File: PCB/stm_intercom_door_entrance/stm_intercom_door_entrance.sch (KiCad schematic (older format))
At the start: 48 parts, among them J1 Conn_01x02, J10 Conn_01x02, J11 Conn_01x04, J12 Conn_01x04, J13 Conn_01x04, J14 Conn_01x02, J15 Conn_01x02, J16 Conn_01x01, J17 Conn_01x03, J18 Conn_01x03, J19 Conn_01x03, J2 Conn_01x04, J3 Conn_01x04, J4 Conn_01x02, J5 Conn_01x04, J6 Conn_01x02, J7 Conn_01x02, J8 Conn_01x04, J9 Conn_01x04, K1 SANYOU_SRD_Form_C, K2 SANYOU_SRD_Form_C, Q1 2N2219, Q2 2N2219, U1 YAAJ_BluePill_Part_Like, U2 MCP2551-I-P, U3 MAX3232_convertor, U4 4N25, U5 L7805, U6 4N25

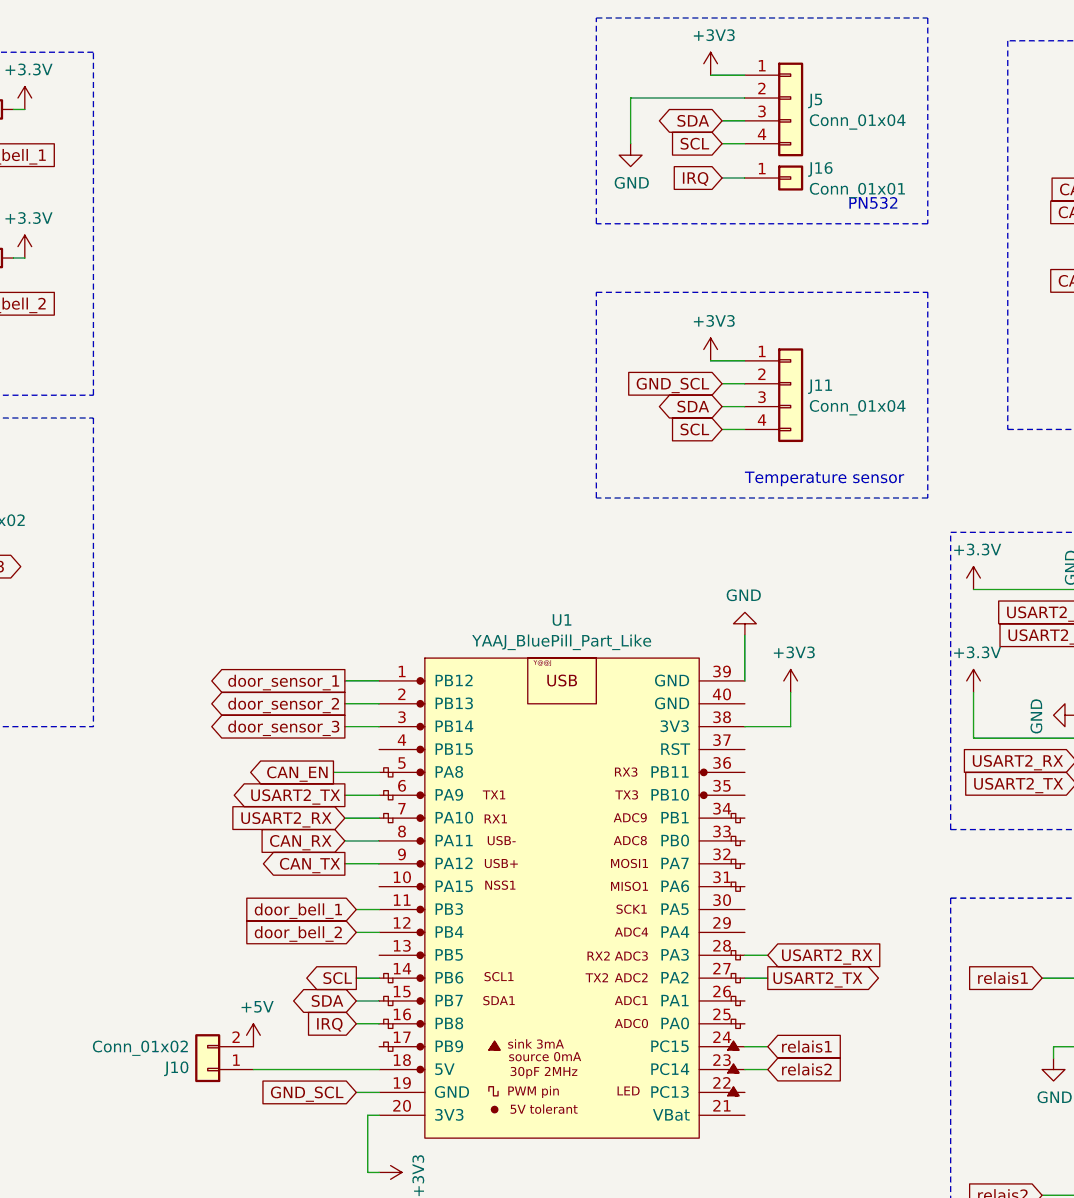
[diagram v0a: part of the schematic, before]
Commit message: Update schematic
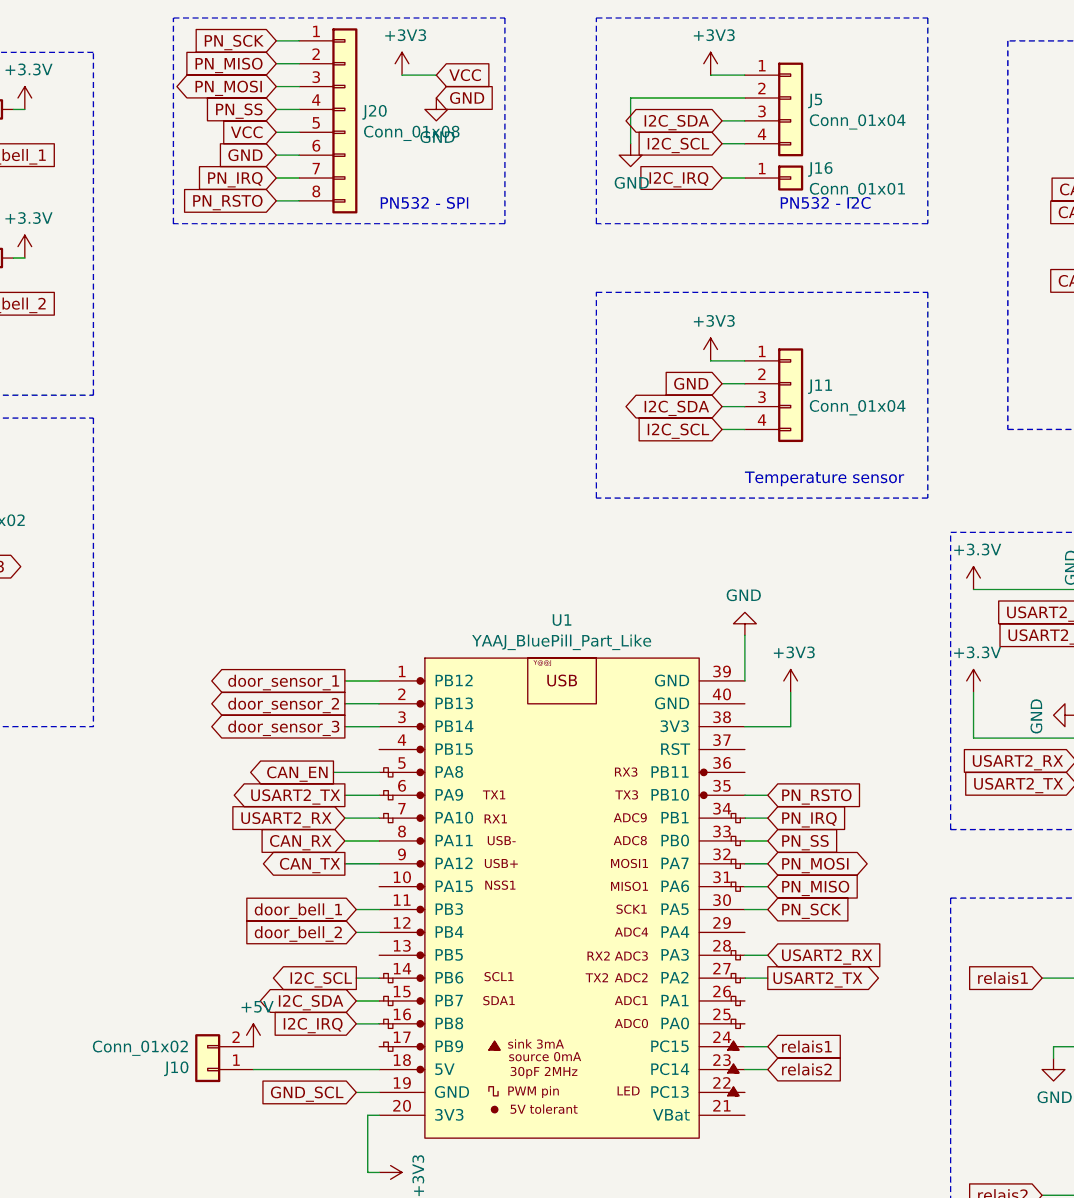
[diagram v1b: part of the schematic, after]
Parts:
- added J20: Conn_01x08, Connector_PinHeader_2.54mm:PinHeader_1x08_P2.54mm_Vertical, symbol Connector_Generic:Conn_01x08
- D2, D3: footprint Diode_THT:Diode_Bridge_DIP-4_W7.62mm_P5.08mm -> Diode_THT:D_5W_P10.16mm_Horizontal
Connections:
- net +3V3: now also J20.5 (Pin_5)
- net GND: now also J11.2 (Pin_2), J20.6 (Pin_6)
- net GND_SCL: no longer J11.2 (Pin_2)
- net PN_SCK: now reaches U1.30 (PA5)
- net PN_SCK: now also J20.1 (Pin_1)
- net PN_MISO: now reaches U1.31 (PA6)
- net PN_MISO: now also J20.2 (Pin_2)
- net PN_MOSI: now reaches U1.32 (PA7)
- net PN_MOSI: now also J20.3 (Pin_3)
- net PN_SS: now reaches U1.33 (PB0)
- net PN_SS: now also J20.4 (Pin_4)
- net PN_IRQ: now reaches U1.34 (PB1)
- net PN_IRQ: now also J20.7 (Pin_7)
- net PN_RSTO: now reaches U1.35 (PB10)
- net PN_RSTO: now also J20.8 (Pin_8)
- net IRQ renamed I2C_IRQ
- net SCL renamed I2C_SCL
- net SDA renamed I2C_SDA
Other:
- note added: "PN532 - I2C"
- note added: "PN532 - SPI"
- note removed: "PN532"
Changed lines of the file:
@@
 $EndComp
 Text GLabel 6400 1050 0    50   BiDi ~ 0
-SDA
+I2C_SDA
 Text GLabel 6400 1150 0    50   Input ~ 0
-SCL
+I2C_SCL
 Wire Wire Line
 	6500 850  6350 850
@@
 	6400 1150 6500 1150
 Text GLabel 4800 4900 0    50   BiDi ~ 0
-SDA
+I2C_SDA
 Wire Wire Line
 	4900 4900 4800 4900
 Text GLabel 4800 4800 0    50   Output ~ 0
-SCL
+I2C_SCL
 Wire Wire Line
 	4900 4800 4800 4800
@@
 	1    0    0    -1
 $EndComp
-Text Notes 6950 1450 0    50   ~ 0
-PN532
+Text Notes 6650 1450 0    50   ~ 0
+PN532 - I2C
 Wire Notes Line
 	7300 600  7300 1500
@@
 $EndComp
 Text GLabel 6400 2300 0    50   BiDi ~ 0
-SDA
+I2C_SDA
 Text GLabel 6400 2400 0    50   Input ~ 0
-SCL
+I2C_SCL
 Wire Wire Line
 	6500 2100 6350 2100
@@
 	6500 3300 6500 3500
 Text GLabel 6400 2200 0    50   Input ~ 0
-GND_SCL
+GND
 Wire Wire Line
 	6400 2200 6500 2200
@@
 $EndComp
 Text GLabel 6400 1300 0    50   Input ~ 0
-IRQ
+I2C_IRQ
 Wire Wire Line
 	6400 1300 6500 1300
 Text GLabel 4800 5000 0    50   Input ~ 0
-IRQ
+I2C_IRQ
 Connection ~ 800  3100
 Connection ~ 1750 3100
@@
 F 0 "D2" H 8700 5167 50  0000 C CNN
 F 1 "D" H 8700 5076 50  0000 C CNN
-F 2 "Diode_THT:Diode_Bridge_DIP-4_W7.62mm_P5.08mm" H 8700 4950 50  0001 C CNN
+F 2 "Diode_THT:D_5W_P10.16mm_Horizontal" H 8700 4950 50  0001 C CNN
 F 3 "~" H 8700 4950 50  0001 C CNN
 	1    8700 4950
@@
 F 0 "D3" H 8700 6117 50  0000 C CNN
 F 1 "D" H 8700 6026 50  0000 C CNN
-F 2 "Diode_THT:Diode_Bridge_DIP-4_W7.62mm_P5.08mm" H 8700 5900 50  0001 C CNN
+F 2 "Diode_THT:D_5W_P10.16mm_Horizontal" H 8700 5900 50  0001 C CNN
 F 3 "~" H 8700 5900 50  0001 C CNN
 	1    8700 5900
@@
 Wire Wire Line
 	4750 3700 4900 3700
+$Comp
+L power:+3V3 #PWR0130
+U 1 1 5FA806A7
+P 5000 850
+F 0 "#PWR0130" H 5000 700 50  0001 C CNN
+F 1 "+3V3" H 5015 1023 50  0000 C CNN
+F 2 "" H 5000 850 50  0001 C CNN
+F 3 "" H 5000 850 50  0001 C CNN
+	1    5000 850
+	1    0    0    -1
+$EndComp
+$Comp
+L power:GND #PWR0131
+U 1 1 5FA806AD
+P 5150 950
+F 0 "#PWR0131" H 5150 700 50  0001 C CNN
+F 1 "GND" H 5155 777 50  0000 C CNN
+F 2 "" H 5150 950 50  0001 C CNN
+F 3 "" H 5150 950 50  0001 C CNN
+	1    5150 950
+	1    0    0    -1
+$EndComp
+Text GLabel 4450 900  0    50   BiDi ~ 0
+PN_MOSI
+Text GLabel 4450 800  0    50   Input ~ 0
+PN_MISO
+Wire Notes Line
+	5450 600  5450 1500
+Wire Notes Line
+	5450 1500 4000 1500
+Wire Notes Line
+	4000 1500 4000 600
+Wire Notes Line
+	4000 600  5450 600
+Text GLabel 4450 1000 0    50   Input ~ 0
+PN_SS
+Text GLabel 4450 700  0    50   Input ~ 0
+PN_SCK
+Text GLabel 4450 1300 0    50   Input ~ 0
+PN_IRQ
+Text GLabel 4450 1200 0    50   Input ~ 0
+GND
+Text GLabel 4450 1400 0    50   Input ~ 0
+PN_RSTO
+$Comp
+L Connector_Generic:Conn_01x08 J20
+U 1 1 5FB1BDFB
+P 4750 1000
+F 0 "J20" H 4830 992 50  0000 L CNN
+F 1 "Conn_01x08" H 4830 901 50  0000 L CNN
+F 2 "Connector_PinHeader_2.54mm:PinHeader_1x08_P2.54mm_Vertical" H 4750 1000 50  0001 C CNN
+F 3 "~" H 4750 1000 50  0001 C CNN
+	1    4750 1000
+	1    0    0    -1
+$EndComp
+Wire Wire Line
+	4450 700  4550 700
+Wire Wire Line
+	4450 800  4550 800
+Wire Wire Line
+	4450 900  4550 900
+Wire Wire Line
+	4450 1000 4550 1000
+Wire Wire Line
+	4450 1200 4550 1200
+Wire Wire Line
+	4450 1300 4550 1300
+Wire Wire Line
+	4450 1400 4550 1400
+Wire Wire Line
+	4450 1100 4550 1100
+Wire Wire Line
+	5150 850  5000 850
+Text GLabel 4450 1100 0    50   Input ~ 0
+VCC
+Text GLabel 5150 850  2    50   Input ~ 0
+VCC
+Text GLabel 5150 950  2    50   Input ~ 0
+GND
+Text Notes 4900 1450 0    50   ~ 0
+PN532 - SPI
+Text GLabel 6600 4300 2    50   BiDi ~ 0
+PN_MOSI
+Text GLabel 6600 4400 2    50   Input ~ 0
+PN_MISO
+Text GLabel 6600 4500 2    50   Input ~ 0
+PN_SCK
+Text GLabel 6600 4100 2    50   Input ~ 0
+PN_IRQ
+Text GLabel 6600 4000 2    50   Input ~ 0
+PN_RSTO
+Wire Wire Line
+	6600 4500 6500 4500
+Wire Wire Line
+	6600 4400 6500 4400
+Wire Wire Line
+	6600 4300 6500 4300
+Wire Wire Line
+	6600 4200 6500 4200
+Wire Wire Line
+	6600 4100 6500 4100
+Wire Wire Line
+	6600 4000 6500 4000
+Text GLabel 6600 4200 2    50   Input ~ 0
+PN_SS
 $EndSCHEMATC

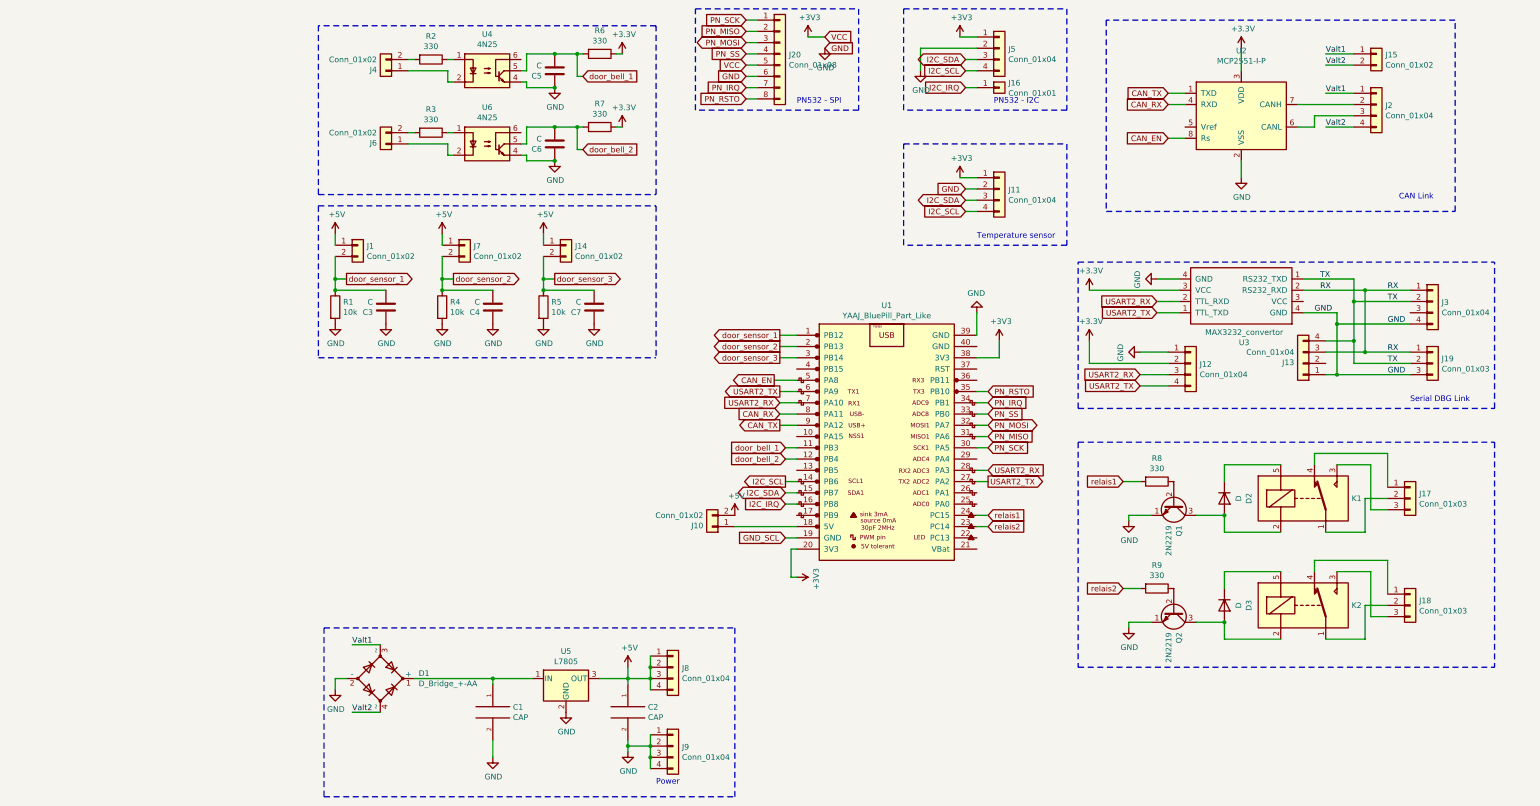
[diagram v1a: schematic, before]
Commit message: update schematics
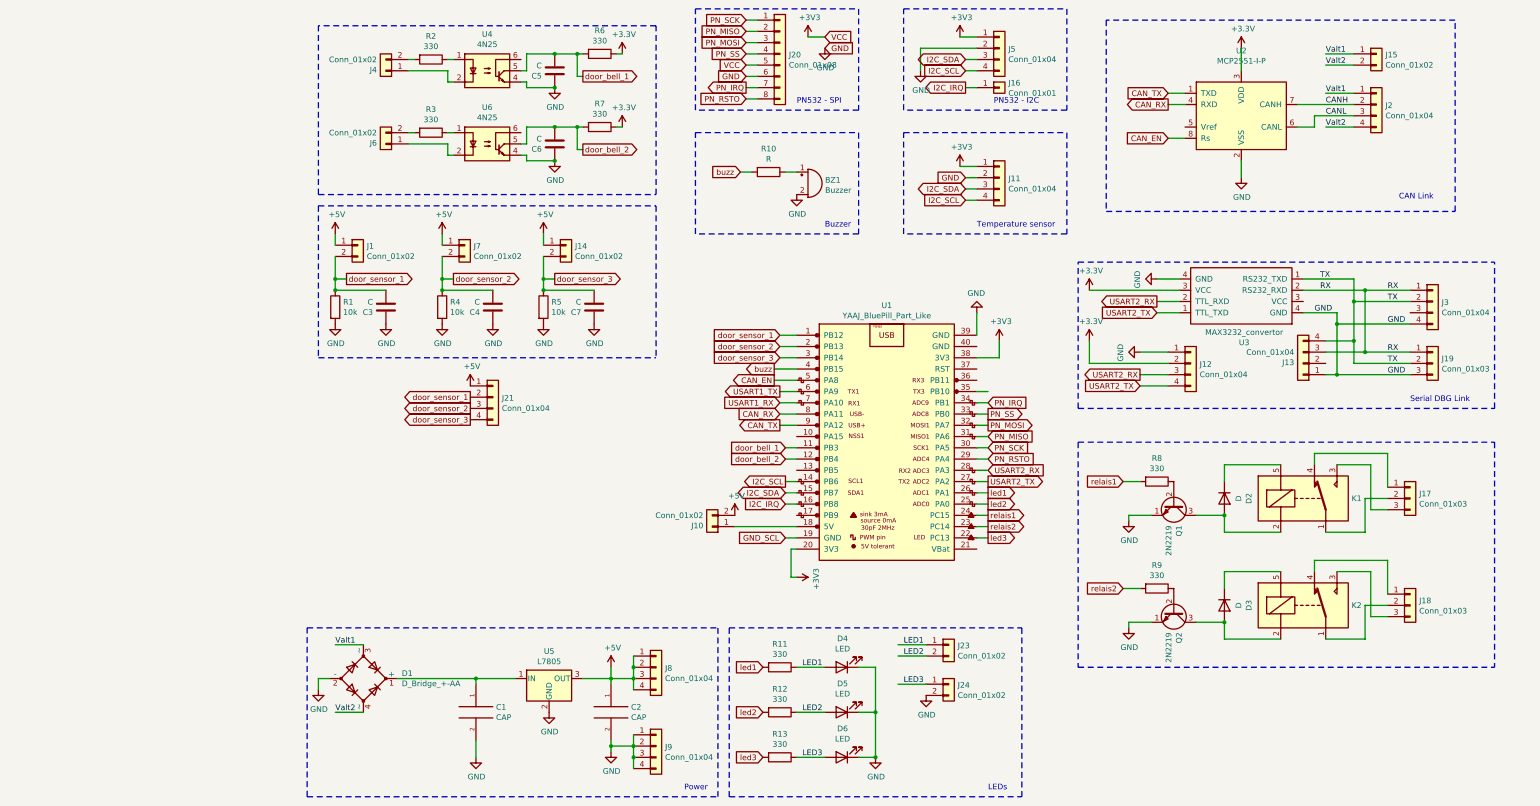
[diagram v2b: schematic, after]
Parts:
- added BZ1: Buzzer, Buzzer_Beeper:Buzzer_12x9.5RM7.6, symbol Device:Buzzer
- added D4, D5, D6: LED, symbol Device:LED
- added J21: Conn_01x04, Connector_PinHeader_2.54mm:PinHeader_1x04_P2.54mm_Vertical, symbol Connector_Generic:Conn_01x04
- added J23, J24: Conn_01x02, Connector_PinHeader_2.54mm:PinHeader_1x02_P2.54mm_Vertical, symbol Connector_Generic:Conn_01x02
- added R10: R, Resistor_THT:R_Axial_DIN0204_L3.6mm_D1.6mm_P7.62mm_Horizontal, symbol Device:R
- added R11, R12, R13: 330, Resistor_THT:R_Axial_DIN0204_L3.6mm_D1.6mm_P5.08mm_Vertical, symbol Device:R
- J3: footprint Connector_PinHeader_2.54mm:PinHeader_1x04_P2.54mm_Horizontal -> Connector_PinHeader_2.54mm:PinHeader_1x04_P2.54mm_Vertical
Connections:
- net +5V: now also J21.1 (Pin_1)
- net GND: now also BZ1.2 (+), D4.1 (K), D5.1 (K), D6.1 (K), J24.2 (Pin_2)
- net PN_RSTO: now also U1.29 (PA4); no longer U1.35 (PB10)
- net USART2_RX: no longer U1.7 (PA10)
- net USART2_TX: no longer U1.6 (PA9)
- net door_sensor_1: now also J21.2 (Pin_2)
- net door_sensor_2: now also J21.3 (Pin_3)
- net door_sensor_3: now also J21.4 (Pin_4)
- net CANL: now reaches J2.3 (Pin_3), U2.6 (CANL)
- net CANH: now reaches J2.2 (Pin_2), U2.7 (CANH)
- net led3: now reaches U1.22 (PC13)
- net led3: now also R13.2
- net led2: now reaches U1.25 (PA0)
- net led2: now also R12.2
- net led1: now reaches U1.26 (PA1)
- net led1: now also R11.2
- net buzz: now reaches U1.4 (PB15)
- net buzz: now also R10.2
- new net: BZ1.1 (-), R10.1
- new net LED1: D4.2 (A), J23.1 (Pin_1), R11.1
- new net LED2: D5.2 (A), J23.2 (Pin_2), R12.1
- new net LED3: D6.2 (A), J24.1 (Pin_1), R13.1
- new net USART1_RX: U1.7 (PA10)
- new net USART1_TX: U1.6 (PA9)
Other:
- note added: "Buzzer"
- note added: "LEDs"
- moved on the sheet: C1, C2, D1, J11, J8, J9, U5

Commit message: Update PCB
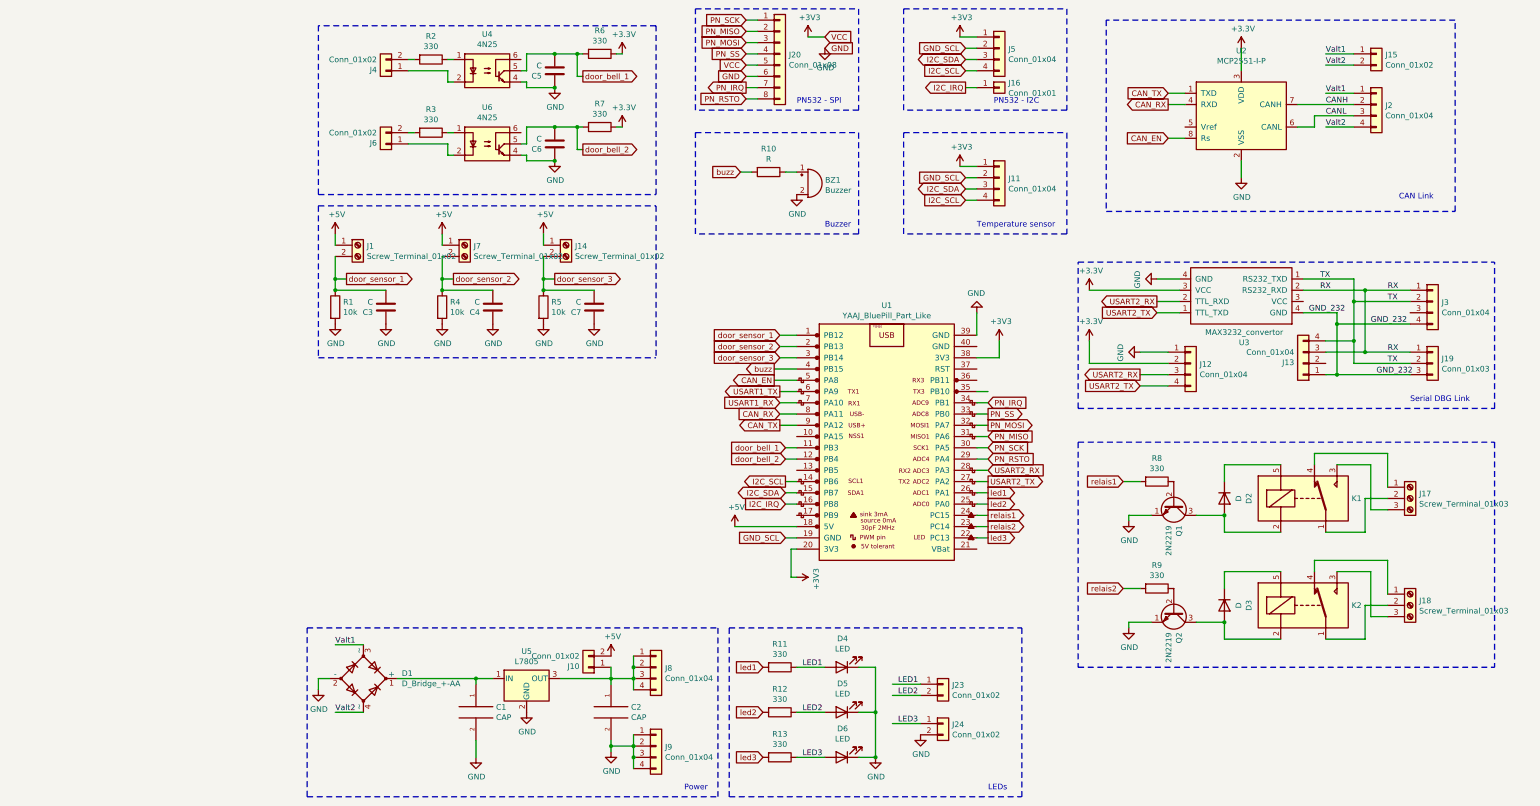
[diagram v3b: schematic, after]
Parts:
- removed J1, J14, J7: Conn_01x02, Connector_PinHeader_2.54mm:PinHeader_1x02_P2.54mm_Vertical, symbol Connector_Generic:Conn_01x02
- removed J17, J18: Conn_01x03, Connector_PinHeader_2.54mm:PinHeader_1x03_P2.54mm_Vertical, symbol Connector_Generic:Conn_01x03
- removed J21: Conn_01x04, Connector_PinHeader_2.54mm:PinHeader_1x04_P2.54mm_Vertical, symbol Connector_Generic:Conn_01x04
- added J1, J14, J7: Screw_Terminal_01x02, TerminalBlock_TE-Connectivity:TerminalBlock_TE_282834-2_1x02_P2.54mm_Horizontal, symbol Connector:Screw_Terminal_01x02
- added J17, J18: Screw_Terminal_01x03, TerminalBlock_TE-Connectivity:TerminalBlock_TE_282834-3_1x03_P2.54mm_Horizontal, symbol Connector:Screw_Terminal_01x03
- C3, C4, C7: footprint Capacitor_THT:CP_Radial_D5.0mm_P2.50mm -> Capacitor_THT:C_Disc_D4.3mm_W1.9mm_P5.00mm
- R10: footprint Resistor_THT:R_Axial_DIN0204_L3.6mm_D1.6mm_P7.62mm_Horizontal -> Resistor_THT:R_Axial_DIN0204_L3.6mm_D1.6mm_P2.54mm_Vertical
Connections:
- net +5V: now also U1.18 (5V), J1.1 (Pin_1), J14.1 (Pin_1), J7.1 (Pin_1); no longer C2.1, J8.1 (Pin_1), J8.2 (Pin_2), J8.3 (Pin_3), J8.4 (Pin_4), U5.3 (OUT)
- net GND: no longer J11.2 (Pin_2), J13.1 (Pin_1), J19.3 (Pin_3), J3.4 (Pin_4), J5.2 (Pin_2)
- net GND_SCL: now also J11.2 (Pin_2), J5.2 (Pin_2)
- net door_sensor_1: now also J1.2 (Pin_2)
- net door_sensor_2: now also J7.2 (Pin_2)
- net door_sensor_3: now also J14.2 (Pin_2)
- net at J10.1 (Pin_1): now also C2.1, J8.1 (Pin_1), J8.2 (Pin_2), J8.3 (Pin_3), J8.4 (Pin_4), U5.3 (OUT); no longer U1.18 (5V)
- net at K1.1: now also J17.2 (Pin_2)
- net at K1.3: now also J17.3 (Pin_3)
- net at K1.4: now also J17.1 (Pin_1)
- net at K2.1: now also J18.2 (Pin_2)
- net at K2.3: now also J18.3 (Pin_3)
- net at K2.4: now also J18.1 (Pin_1)
- new net GND_232: J13.1 (Pin_1), J19.3 (Pin_3), J3.4 (Pin_4), U3.4 (GND)
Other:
- moved on the sheet: J10, J23, J24, U5
